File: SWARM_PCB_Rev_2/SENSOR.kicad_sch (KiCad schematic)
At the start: 15 parts

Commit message: Updated Via size to 0.25mm and ReExported Files
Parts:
- cC1, cC2, cC3, cC4, cC5, cC6, cC7, cC8, cC9: Manufacturer Murata -> (none)
- cR1, cR2: Manufacturer Yageo -> (none)
- cU1: Manufacturer MEMSIC -> (none)
- cU2: Manufacturer STMicroelectronics -> (none)
- cU3: Manufacturer TE Connectivity -> (none)
- cU4: Availability In Stock -> (none); Manufacturer STMicroelectronics -> (none); Package VFLGA-14 STMicroelectronics -> (none); Price None -> (none)
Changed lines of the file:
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@@
 			)
 		)
-		(property "Manufacturer" "MEMSIC"
-			(at 0 0 0)
-			(hide yes)
-			(show_name no)
-			(do_not_autoplace no)
-			(effects
-				(font
-					(size 1.27 1.27)
-				)
-			)
-		)
 		(property "MPN" "MMC5603NJ"
 			(at 0 0 0)
@@
 			)
 		)
-		(property "Manufacturer" "Murata"
-			(at 49.53 -12.7 0)
-			(hide yes)
-			(show_name no)
-			(do_not_autoplace no)
-			(effects
-				(font
-					(size 1.27 1.27)
-				)
-			)
-		)
 		(property "MPN" "GRM188R60J106ME47D"
 			(at 49.53 -12.7 0)
@@
 			)
 		)
-		(property "Manufacturer" "Murata"
-			(at 0 0 0)
-			(hide yes)
-			(show_name no)
-			(do_not_autoplace no)
-			(effects
-				(font
-					(size 1.27 1.27)
-				)
-			)
-		)
 		(property "MPN" "GRM188R71C104KA01D"
 			(at 0 0 0)
@@
 			)
 		)
-		(property "Manufacturer" "Yageo"
-			(at 0 0 0)
-			(hide yes)
-			(show_name no)
-			(do_not_autoplace no)
-			(effects
-				(font
-					(size 1.27 1.27)
-				)
-			)
-		)
 		(property "MPN" "RC0603FR-072K2L"
 			(at 0 0 0)
@@
 			)
 		)
-		(property "Manufacturer" "STMicroelectronics"
-			(at 0 0 0)
-			(hide yes)
-			(show_name no)
-			(do_not_autoplace no)
-			(effects
-				(font
-					(size 1.27 1.27)
-				)
-			)
-		)
 		(property "MPN" "ASM330LHHXTR"
 			(at 0 0 0)
@@
 			)
 		)
-		(property "Package" "VFLGA-14 STMicroelectronics"
-			(at 43.18 76.2 0)
-			(hide yes)
-			(show_name no)
-			(do_not_autoplace no)
-			(effects
-				(font
-					(size 1.27 1.27)
-				)
-				(justify bottom)
-			)
-		)
-		(property "Price" "None"
-			(at 43.18 76.2 0)
-			(hide yes)
-			(show_name no)
-			(do_not_autoplace no)
-			(effects
-				(font
-					(size 1.27 1.27)
-				)
-				(justify bottom)
-			)
-		)
-		(property "Availability" "In Stock"
-			(at 43.18 76.2 0)
-			(hide yes)
-			(show_name no)
-			(do_not_autoplace no)
-			(effects
-				(font
-					(size 1.27 1.27)
-				)
-				(justify bottom)
-			)
-		)
-		(property "Manufacturer" "STMicroelectronics"
-			(at 0 0 0)
-			(hide yes)
-			(show_name no)
-			(do_not_autoplace no)
-			(effects
-				(font
-					(size 1.27 1.27)
-				)
-			)
-		)
 		(property "MPN" "LSM6DSO32TR"
 			(at 0 0 0)
@@
 			)
 		)
-		(property "Manufacturer" "Murata"
-			(at 0 0 0)
-			(hide yes)
-			(show_name no)
-			(do_not_autoplace no)
-			(effects
-				(font
-					(size 1.27 1.27)
-				)
-			)
-		)
 		(property "MPN" "GRM188R71C104KA01D"
 			(at 0 0 0)
@@
 			)
 		)
-		(property "Manufacturer" "Murata"
-			(at 0 0 0)
-			(hide yes)
-			(show_name no)
-			(do_not_autoplace no)
-			(effects
-				(font
-					(size 1.27 1.27)
-				)
-			)
-		)
 		(property "MPN" "GRM188R60J225KE15D"
 			(at 0 0 0)
@@
 			)
 		)
-		(property "Manufacturer" "Murata"
-			(at 0 0 0)
-			(hide yes)
-			(show_name no)
-			(do_not_autoplace no)
-			(effects
-				(font
-					(size 1.27 1.27)
-				)
-			)
-		)
 		(property "MPN" "GRM188R60J106ME47D"
 			(at 0 0 0)
@@
 			)
 		)
-		(property "Manufacturer" "Murata"
-			(at 0 0 0)
-			(hide yes)
-			(show_name no)
-			(do_not_autoplace no)
-			(effects
-				(font
-					(size 1.27 1.27)
-				)
-			)
-		)
 		(property "MPN" "GRM188R71C104KA01D"
 			(at 0 0 0)
@@
 			)
 		)
-		(property "Manufacturer" "Murata"
-			(at 0 0 0)
-			(hide yes)
-			(show_name no)
-			(do_not_autoplace no)
-			(effects
-				(font
-					(size 1.27 1.27)
-				)
-			)
-		)
 		(property "MPN" "GRM188R60J106ME47D"
 			(at 0 0 0)
@@
 			)
 		)
-		(property "Manufacturer" "Murata"
-			(at 0 0 0)
-			(hide yes)
-			(show_name no)
-			(do_not_autoplace no)
-			(effects
-				(font
-					(size 1.27 1.27)
-				)
-			)
-		)
 		(property "MPN" "GRM188R71C104KA01D"
 			(at 0 0 0)
@@
 			)
 		)
-		(property "Manufacturer" "Yageo"
-			(at 0 0 0)
-			(hide yes)
-			(show_name no)
-			(do_not_autoplace no)
-			(effects
-				(font
-					(size 1.27 1.27)
-				)
-			)
-		)
 		(property "MPN" "RC0603FR-072K2L"
 			(at 0 0 0)
@@
 			)
 		)
-		(property "Manufacturer" "Murata"
-			(at 0 0 0)
-			(hide yes)
-			(show_name no)
-			(do_not_autoplace no)
-			(effects
-				(font
-					(size 1.27 1.27)
-				)
-			)
-		)
 		(property "MPN" "GRM188R71C104KA01D"
 			(at 0 0 0)
@@
 			(hide yes)
 			(show_name no)
-			(do_not_autoplace no)
-			(effects
-				(font
-					(size 1.27 1.27)
-				)
-			)
-		)
-		(property "Manufacturer" "TE Connectivity"
-			(at 0 0 0)
-			(hide yes)
-			(show_name no)

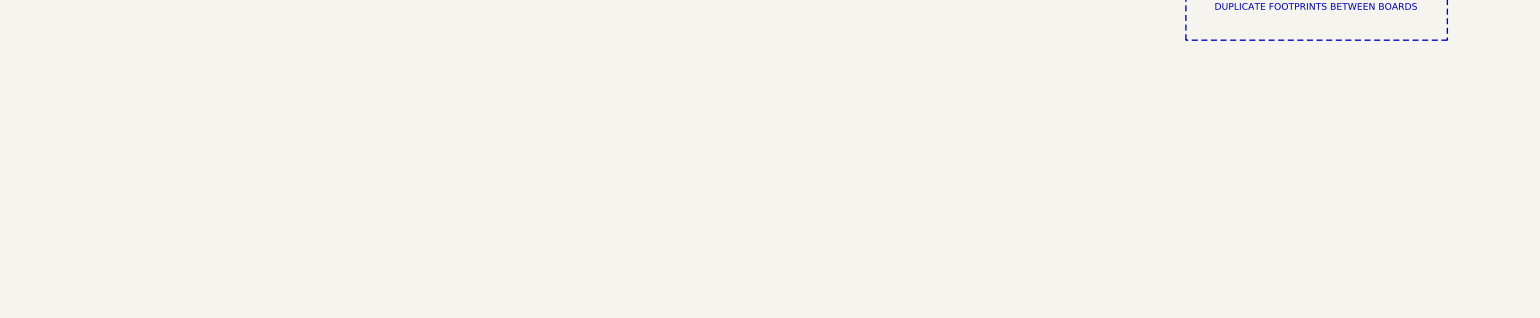
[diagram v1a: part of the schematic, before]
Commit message: Cleaned up Schematic and Exported
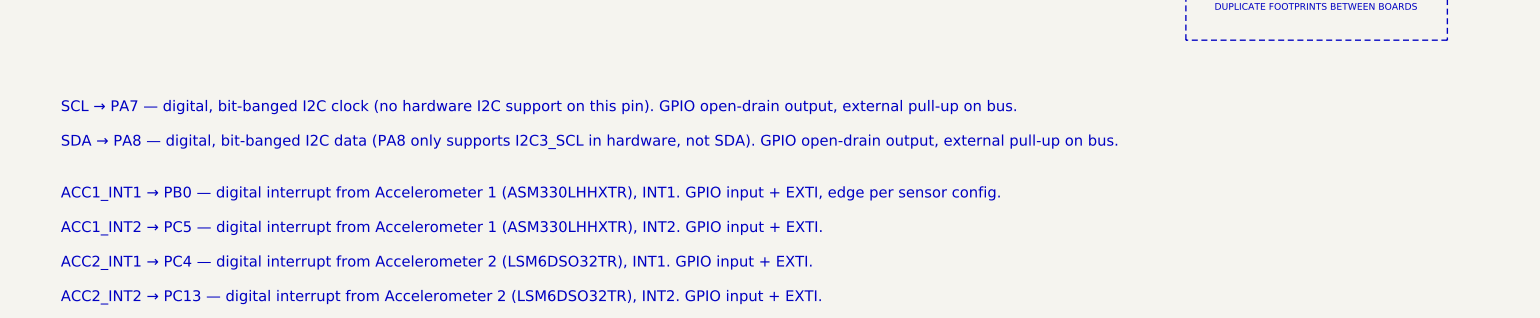
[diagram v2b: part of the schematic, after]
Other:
- note added: "SCL → PA7 — digital, bit-banged I2C clock (no hardware I2C support on this pin). GPIO open-drain output, external pull-up on bus. SDA → PA8 — digital, bit-banged I2C data (PA8 only supports I2C3_SCL in hardware, not SDA). GPIO open-drain output, external pull-up on bus. ACC1_INT1 → PB0 — digital interrupt from Accelerometer 1 (ASM330LHHXTR), INT1. GPIO input + EXTI, edge per sensor config. ACC1_I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"
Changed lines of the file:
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@@
+		)
+	)
+	(text "SCL → PA7 — digital, bit-banged I2C clock (no hardware I2C support on this pin). GPIO open-drain output, external pull-up on bus.\n\nSDA → PA8 — digital, bit-banged I2C data (PA8 only supports I2C3_SCL in hardware, not SDA). GPIO open-drain output, external pull-up on bus.\n\n\nACC1_INT1 → PB0 — digital interrupt from Accelerometer 1 (ASM330LHHXTR), INT1. GPIO input + EXTI, edge per sensor config.\n\nACC1_INT2 → PC5 — digital interrupt from Accelerometer 1 (ASM330LHHXTR), INT2. GPIO input + EXTI.\n\nACC2_INT1 → PC4 — digital interrupt from Accelerometer 2 (LSM6DSO32TR), INT1. GPIO input + EXTI.\n\nACC2_INT2 → PC13 — digital interrupt from Accelerometer 2 (LSM6DSO32TR), INT2. GPIO input + EXTI."
+		(exclude_from_sim no)
+		(at 21.844 134.874 0)
+		(effects
+			(font
+				(size 2.032 2.032)
+			)
+			(justify left)
 		)
 	)
